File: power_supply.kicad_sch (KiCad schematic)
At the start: 17 parts, among them J10 CONN_01X02, J11 CONN_01X02, J8 UJC-HP-3-SMT-TR, J9 5V, Q1 ZXMP6A13FTA, SW1 SW_SPDT, U10 MCP73831, U11 DC-DC-Boost-Converter-Positiv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

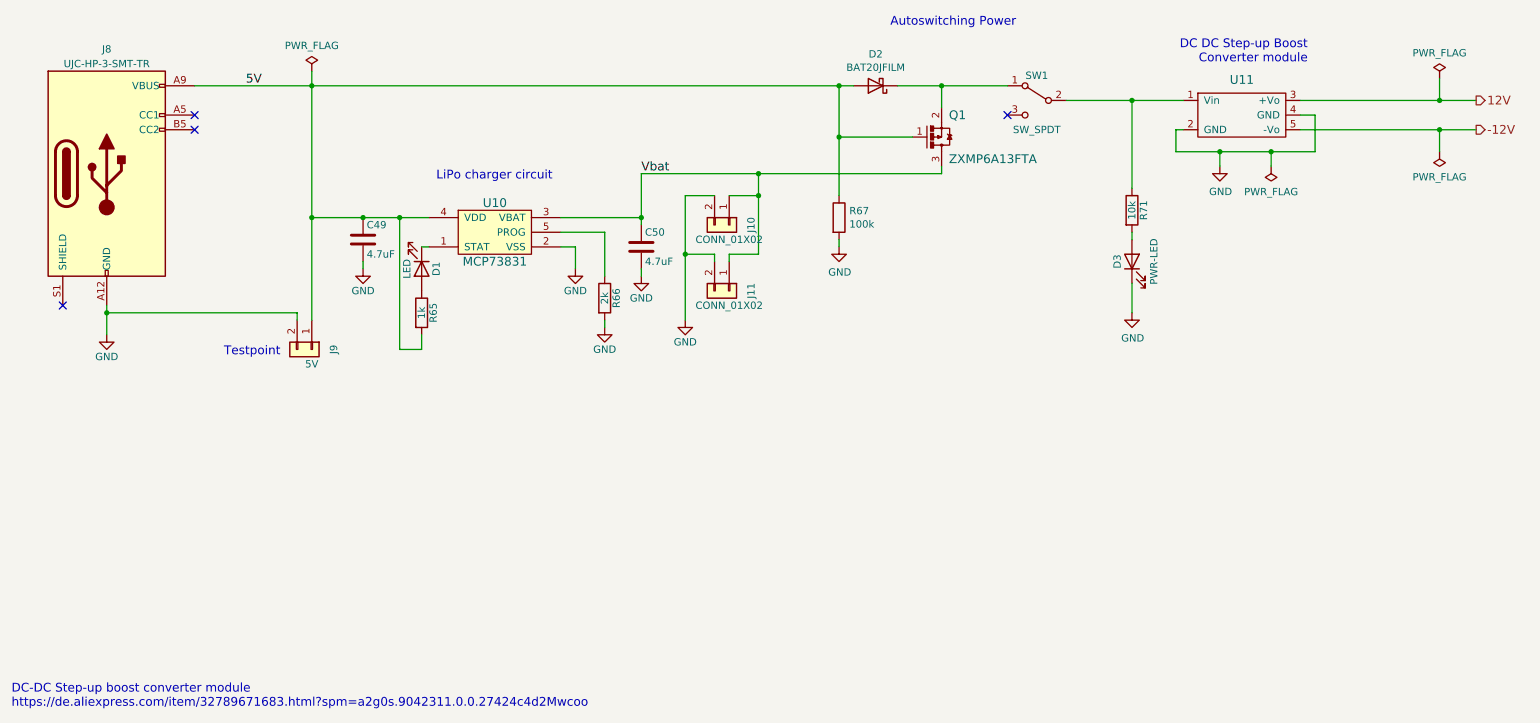
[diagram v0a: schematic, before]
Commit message: documentation / update kicad
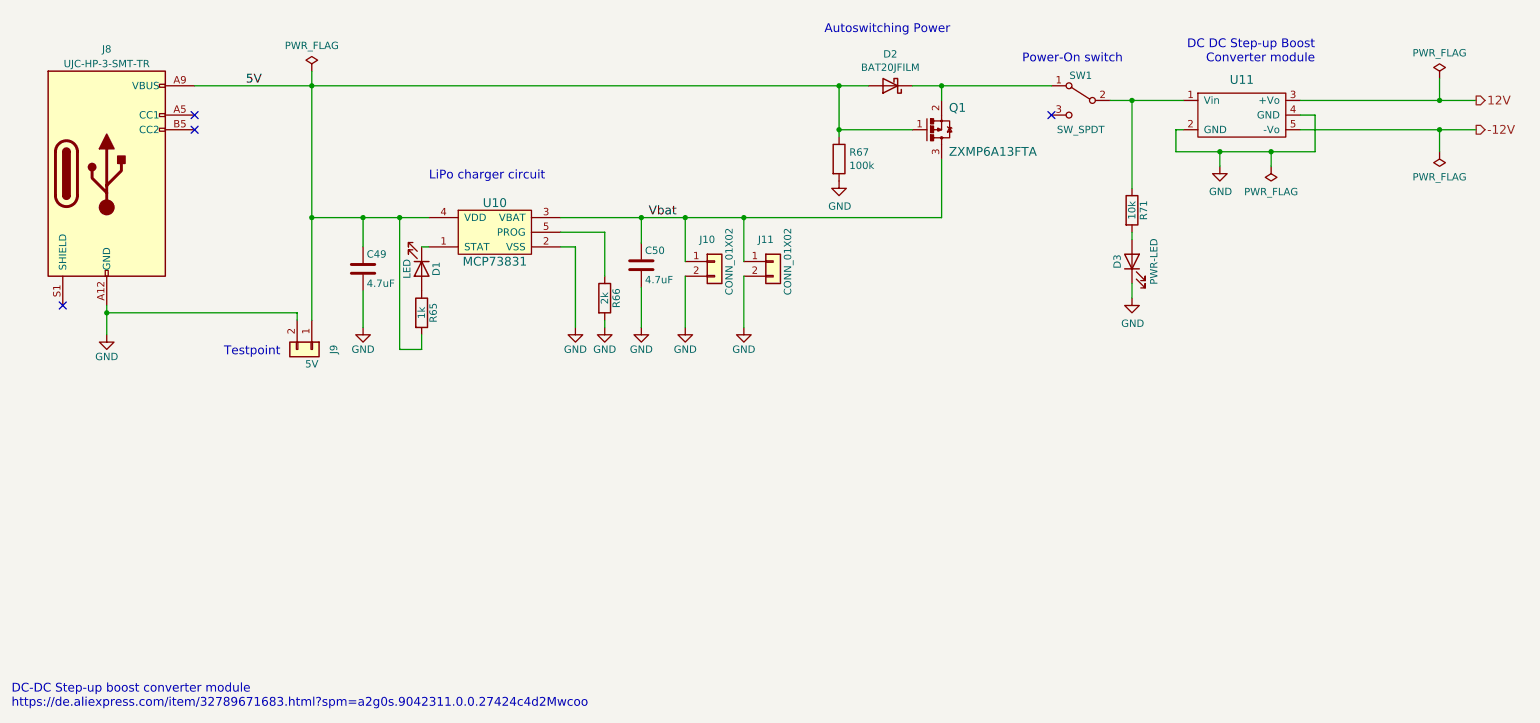
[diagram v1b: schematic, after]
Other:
- note added: "Power-On switch"
- moved on the sheet: C49, C50, D2, J10, J11, Q1, R67, SW1
